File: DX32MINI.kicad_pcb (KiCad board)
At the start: 2 copper layers, 25.4 x 47.6 mm, 19 parts, among them J1 USB_B_Micro, J2 MicroSD Card, J3 GPIO - Left, J4 GPIO - Right, J5 Reset and Boot pins, SW1 reset, SW2 boot, U1 ESP32-S3-WROOM-1, U2 AMS1117-3.3

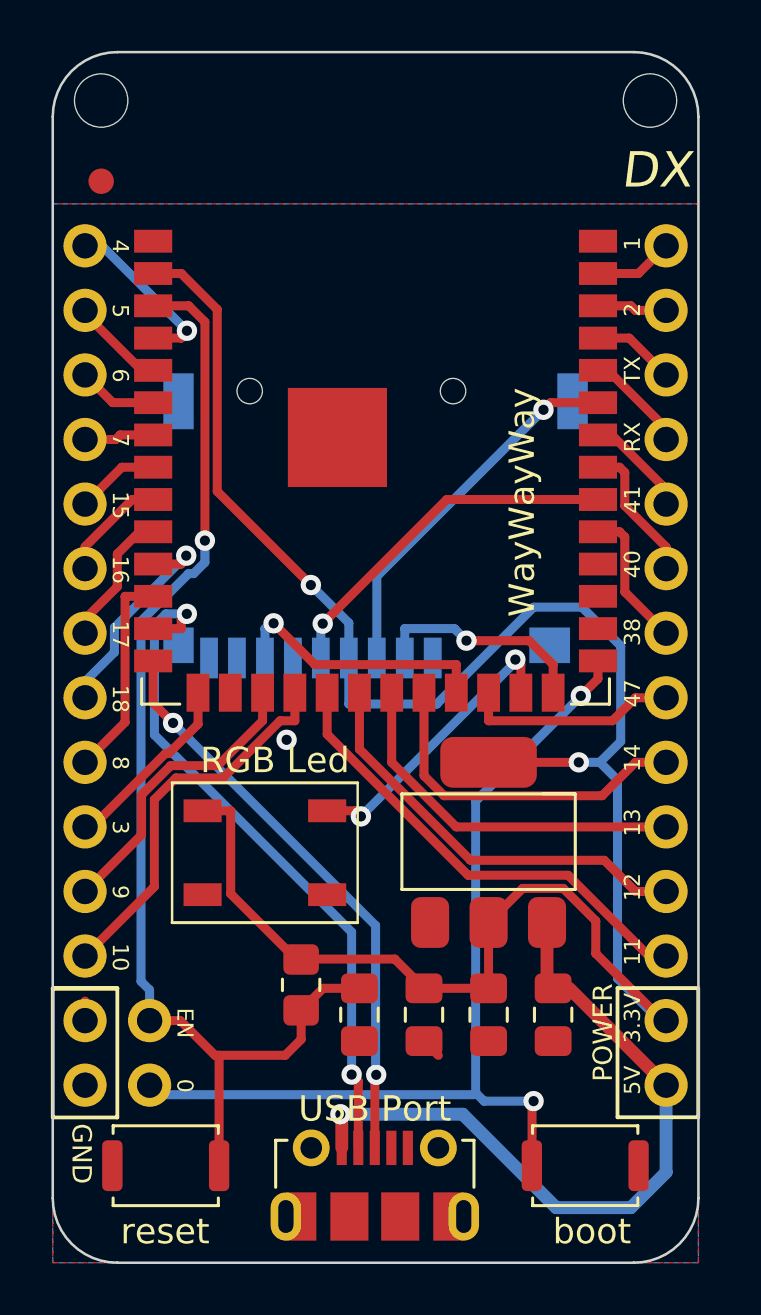
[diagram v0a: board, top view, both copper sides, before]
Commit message: Add files via upload
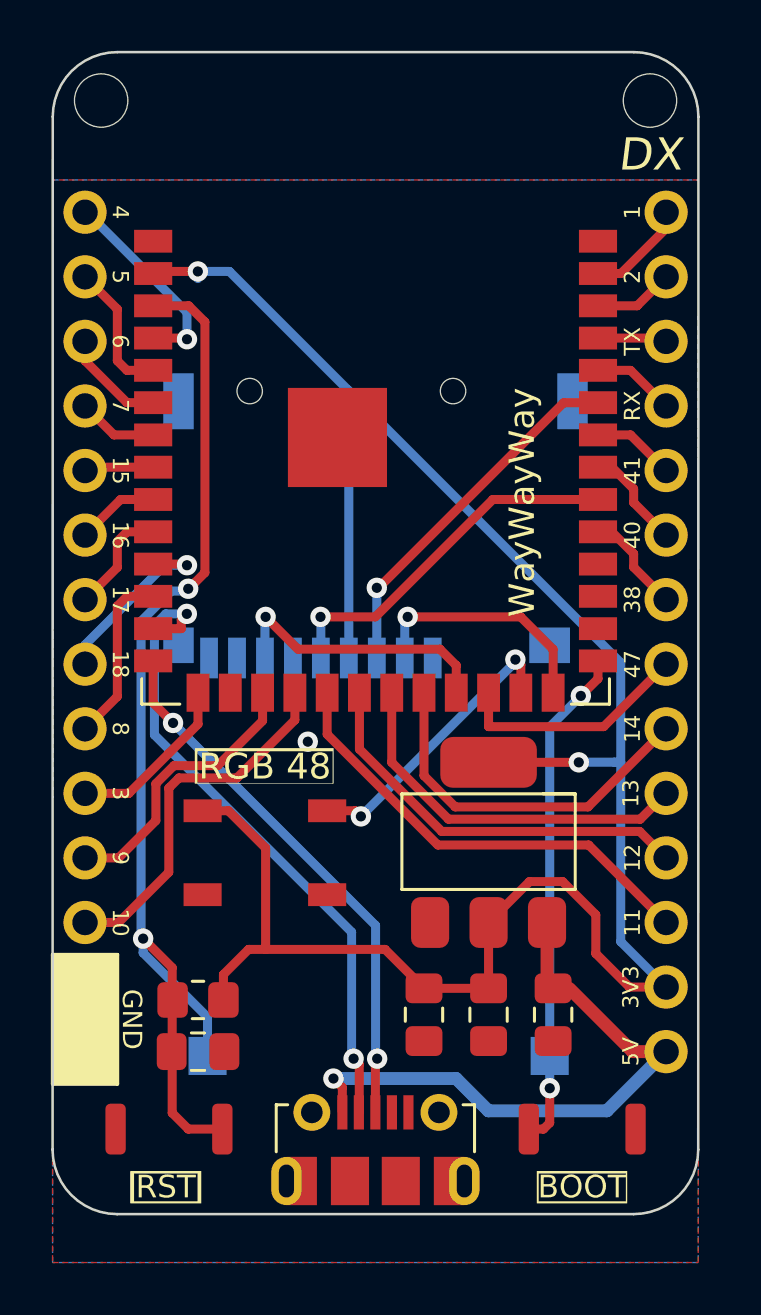
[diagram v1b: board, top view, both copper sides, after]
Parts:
- removed J5: Reset and Boot pins, Connector_PinHeader_2.54mm:PinHeader_1x02_P2.54mm_Vertical
- removed fid: Fiducial_1mm_Mask2mm, Fiducial:Fiducial_1mm_Mask2mm
- added TP1: RESET, TestPoint:TestPoint_Pad_1.5x1.5mm, B.Cu at (183.9, 118.9)
- added TP2: RESET, TestPoint:TestPoint_Pad_1.5x1.5mm, B.Cu at (197.4, 118.9)
- moved C1 6.51 mm to (183.5, 118.7), turned to 0 degrees
- moved R1 4.10 mm to (183.5, 116.7), turned to 180 degrees
- moved SW2 1.45 mm to (182.4, 121.8)
- moved SW1 1.44 mm to (198.6, 121.8)
- moved J1 1.40 mm to (190.5, 122.6)
- moved J3 1.32 mm to (201.9, 118.7)
- moved J2 1.32 mm to (179.1, 85.7)
- moved G*** 1.28 mm to (182.2, 123.2)
- renumbered J3 to J2, J4 to J3, J2 to J4, SW2 to SW1, SW1 to SW2
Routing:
- net /BOOT: track 37.0 -> 20.0 mm
- net GND: track 9.63 -> 5.77 mm
- net +5V: track 27.8 -> 24.1 mm
- net +3.3V: track 83.5 -> 86.8 mm
- net /RESET: track 46.0 -> 43.2 mm, vias 1 -> 2
- net /GPIO5: track 3.73 -> 5.39 mm
- net /GPIO38: track 5.60 -> 4.10 mm
- net /GPIO40: track 5.60 -> 4.10 mm
- net /GPIO8: track 8.29 -> 6.92 mm
- net /GPIO18: track 8.76 -> 7.42 mm
- net /USB_D+: track 22.7 -> 21.4 mm
- net /USB_D-: track 27.0 -> 25.7 mm
- net /GPIO4: track 6.88 -> 8.05 mm
- net /GPIO16: track 4.31 -> 3.26 mm
- net /GPIO17: track 5.42 -> 4.38 mm
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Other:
- board size 25.4 x 47.6 mm -> 25.4 x 45.7 mm
- board text added: "3V3"
- board text added: "BOOT"
- board text added: "DX32A DELUXE Designed In Chile IrregularDX 2024"
- board text added: "RST"
- board text added: "SD"
- board text removed: "0"
- board text removed: "3.3V"
- board text removed: "DX32A DELUXE Mini Open source hardware Designed In Chile IrregularDX 2024"
- board text removed: "EN"
- board text removed: "POWER"
- board text removed: "SD Card"
- board text removed: "rev. 1.2"
